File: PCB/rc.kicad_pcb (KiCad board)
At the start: 2 copper layers, 31.8 x 19 mm, 13 parts, among them J1 Conn_01x03_Pin, J10 Conn_01x03_Pin, J11 Conn_01x03_Pin, J2 Conn_01x03_Pin, J3 Conn_01x03_Pin, J4 Conn_01x03_Pin, J5 Conn_01x03_Pin, J6 Conn_01x03_Pin, J7 Conn_01x03_Pin, J8 Conn_01x03_Pin, J9 Conn_01x03_Pin, P1 USB_C_Plug_USB2.0, U2 ESP32-S3-MINI-1U

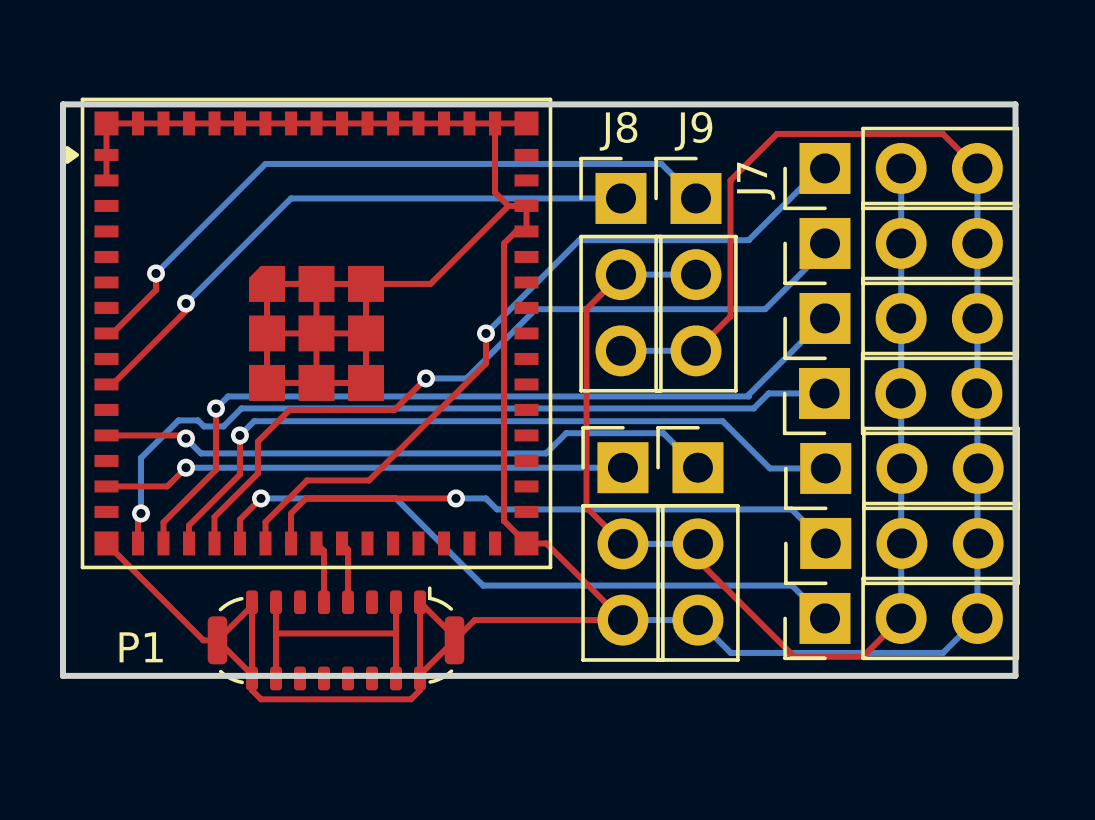
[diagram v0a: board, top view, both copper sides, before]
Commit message: smaller
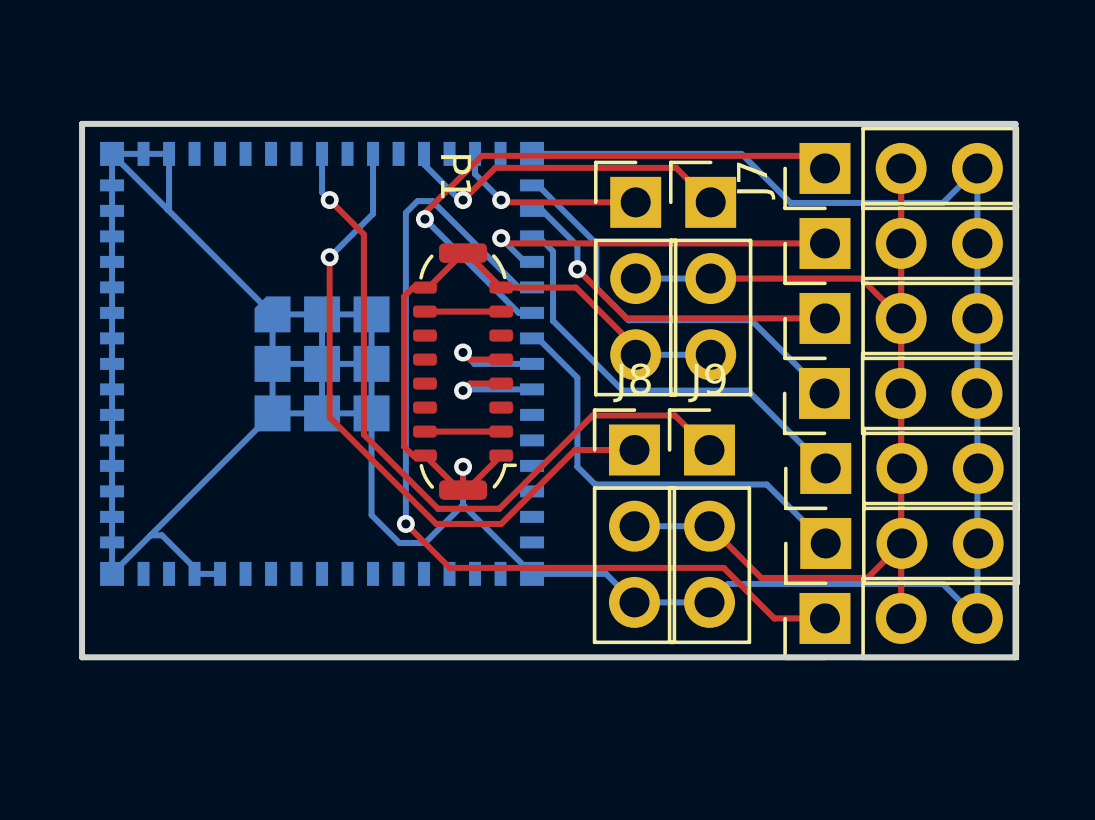
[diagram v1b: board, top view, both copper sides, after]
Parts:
- U2: moved to B.Cu
- moved P1 9.91 mm to (38.7, 129.5), turned to 180 degrees
- moved J10 8.86 mm to (44.5, 123.9)
- moved J11 8.86 mm to (47.0, 123.9)
- moved J8 8.40 mm to (44.5, 132.2)
- moved J9 8.40 mm to (47.0, 132.2)
- moved U2 1.03 mm to (34.0, 129.3), turned to -90 degrees
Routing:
- net Net-(J5-Pin_1): track 26.8 -> 11.7 mm
- net Net-(J6-Pin_1): track 25.8 -> 12.2 mm
- net Net-(J4-Pin_1): track 26.7 -> 13.5 mm, vias 1 -> 0
- net Net-(J10-Pin_1): track 17.5 -> 6.49 mm
- net Net-(J3-Pin_1): track 24.7 -> 14.4 mm, vias 1 -> 0
- net Net-(J11-Pin_1): track 20.7 -> 11.3 mm
- net Net-(J1-Pin_1): track 22.2 -> 31.2 mm
- net Net-(J7-Pin_1): track 24.8 -> 19.4 mm
- net Net-(J2-Pin_1): track 19.7 -> 14.4 mm, vias 1 -> 0
- net Net-(J1-Pin_2): track 39.1 -> 34.5 mm
- net Net-(P1-VBUS-PadA4): track 9.08 -> 5.08 mm
- net Net-(J8-Pin_1): track 19.9 -> 22.0 mm
- net Net-(P1-D-): track 2.06 -> 3.82 mm, vias 0 -> 1
- net Net-(P1-D+): track 2.04 -> 3.68 mm, vias 0 -> 1
- net Net-(J9-Pin_1): track 22.8 -> 24.2 mm
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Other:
- board size 31.8 x 19 mm -> 31.1 x 17.8 mm

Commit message: more components
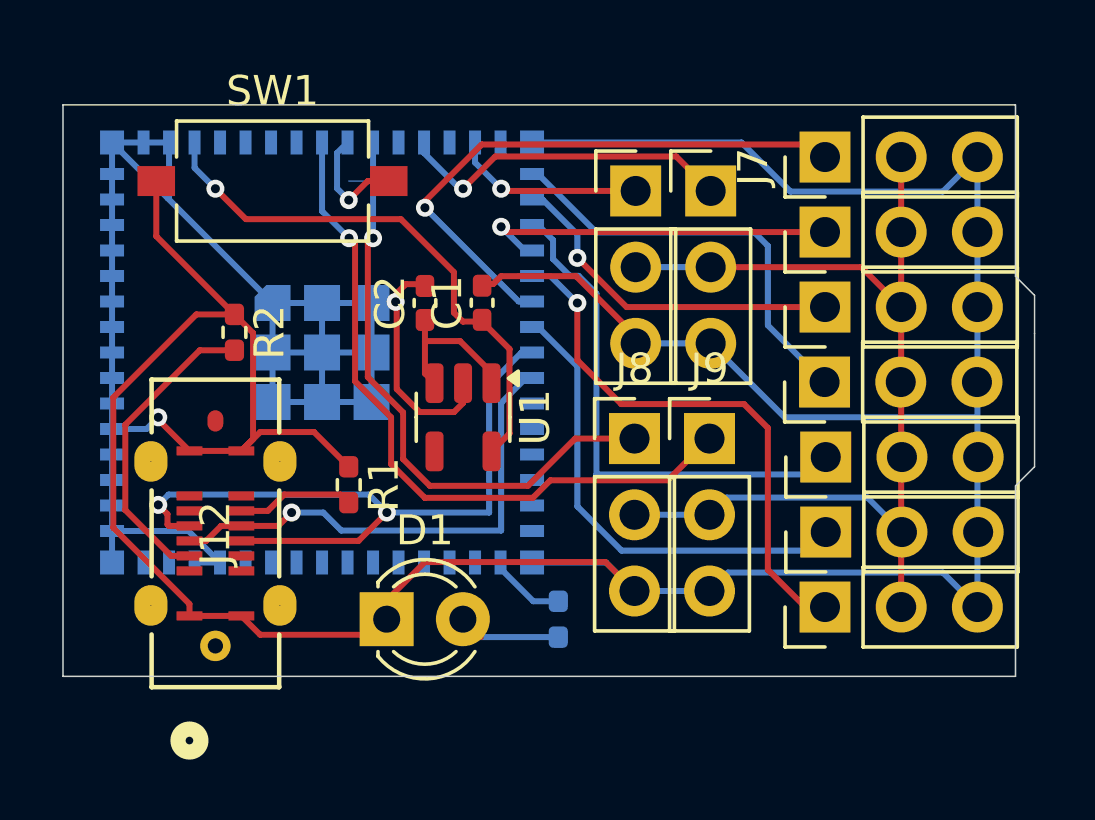
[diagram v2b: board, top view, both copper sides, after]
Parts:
- removed P1: USB_C_Plug_USB2.0, Connector_USB:USB_C_Plug_ShenzhenJingTuoJin_918-118A2021Y40002_Vertical
- added C1: C, Capacitor_SMD:C_0402_1005Metric_Pad0.74x0.62mm_HandSolder, F.Cu at (39.4, 127.2)
- added C2: C, Capacitor_SMD:C_0402_1005Metric_Pad0.74x0.62mm_HandSolder, F.Cu at (37.5, 127.3)
- added D1: LED, LED_THT:LED_D3.0mm, F.Cu at (36.2, 137.8)
- added J12: USB4120-03-C_REVA, usbc:USB4120-03-C_GCT, F.Cu at (29.6, 137.7)
- added R1: R_US, Resistor_SMD:R_0402_1005Metric_Pad0.72x0.64mm_HandSolder, F.Cu at (34.9, 133.3)
- added R2: R_US, Resistor_SMD:R_0402_1005Metric_Pad0.72x0.64mm_HandSolder, F.Cu at (31.1, 128.2)
- added R3: R_US, Resistor_SMD:R_0402_1005Metric_Pad0.72x0.64mm_HandSolder, B.Cu at (41.9, 137.8)
- added SW1: SW_Push, Button_Switch_SMD:SW_Tactile_SPST_NO_Straight_CK_PTS636Sx25SMTRLFS, F.Cu at (32.4, 123.2)
- added U1: ME6211C33M5, Package_TO_SOT_SMD:SOT-23-5, F.Cu at (38.7, 131.1)
- moved J1 0.38 mm to (50.8, 137.4)
- moved J2 0.38 mm to (50.8, 134.9)
- moved J3 0.38 mm to (50.8, 132.4)
- moved J4 0.38 mm to (50.8, 129.9)
- moved J10 0.38 mm to (44.5, 123.5)
- moved J11 0.38 mm to (47.0, 123.5)
- moved J5 0.38 mm to (50.8, 127.4)
- moved J6 0.38 mm to (50.8, 124.9)
- moved J7 0.38 mm to (50.8, 122.4)
- moved J8 0.38 mm to (44.5, 131.8)
- moved J9 0.38 mm to (47.0, 131.8)
- moved U2 0.38 mm to (34.0, 128.9)
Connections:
- U2 pad 3: unconnected-(U2-3V3-Pad3) -> Net-(U1-V_{OUT})
- U2 pad 31: unconnected-(U2-IO35-Pad31) -> Net-(U2-IO35)
- U2 pad 9: unconnected-(U2-IO5-Pad9) -> Net-(U2-IO5)
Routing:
- net Net-(D1-K): track 137.0 -> 175.4 mm, vias 1 -> 2
- net Net-(J12-D1-): track 3.82 -> 24.3 mm, vias 1 -> 2
- net Net-(U1-V_{OUT}): track 0.00 -> 18.3 mm, vias 0 -> 1
- net Net-(J12-D1+): track 3.68 -> 16.7 mm
- net Net-(J1-Pin_1): track 31.2 -> 18.7 mm
- net Net-(J12-CC1): track 0.00 -> 10.3 mm
- net Net-(U1-CE): track 0.00 -> 5.19 mm
- net Net-(P1-VBUS-PadA4): track 5.08 -> 0.00 mm
- net Net-(D1-A): track 0.00 -> 4.27 mm
- net Net-(J12-CC2): track 0.00 -> 3.92 mm
- net Net-(U2-IO5): track 0.00 -> 3.82 mm, vias 0 -> 1
- net Net-(J3-Pin_1): track 14.4 -> 17.4 mm
- net Net-(U2-IO35): track 0.00 -> 2.58 mm
- net Net-(J8-Pin_1): track 22.0 -> 19.8 mm
- net Net-(J2-Pin_1): track 14.4 -> 15.9 mm
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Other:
- board size 31.1 x 17.8 mm -> 32.4 x 19 mm
